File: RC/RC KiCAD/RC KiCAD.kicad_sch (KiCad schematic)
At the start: 10 parts, among them J1 USB_C_Receptacle_PowerOnly_6P, U1 MCP73871, U2 CR2013-MI2120

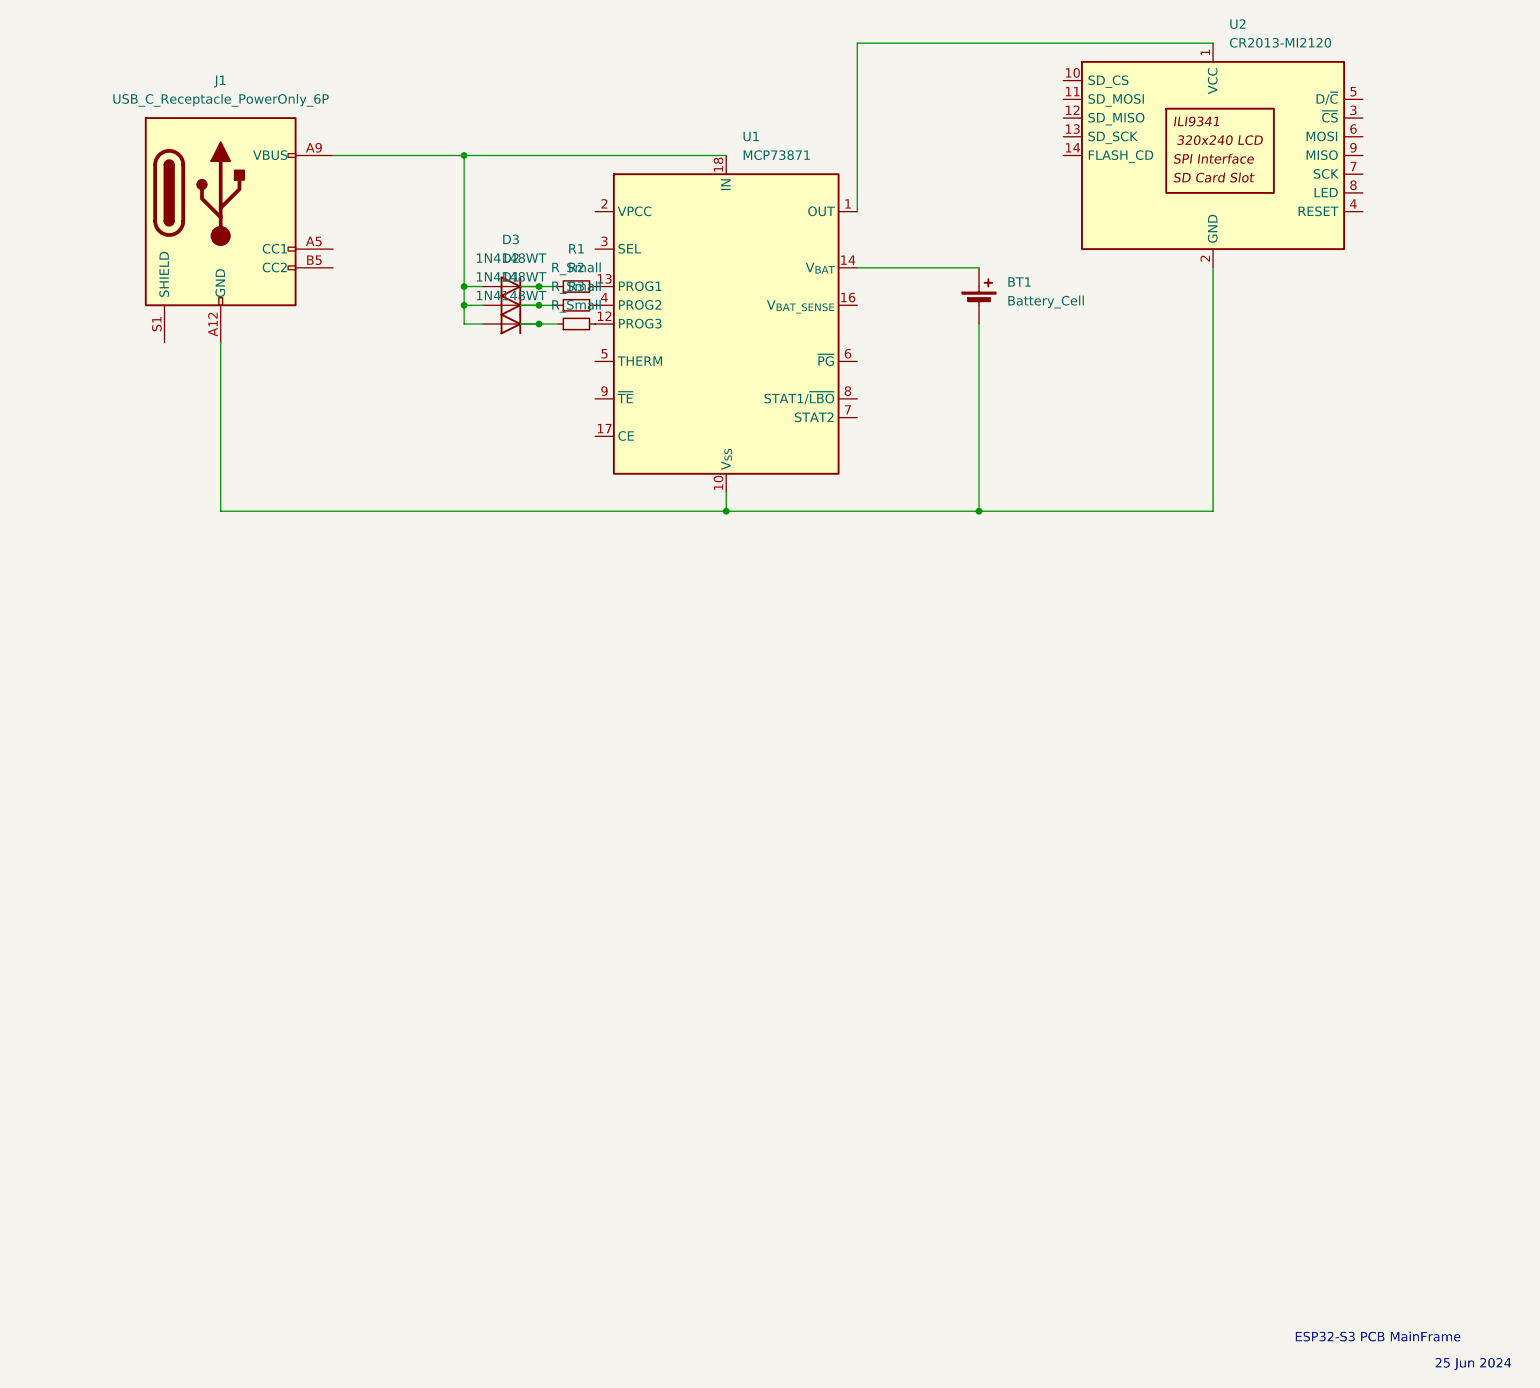
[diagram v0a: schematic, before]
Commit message: BMS FULL CAO
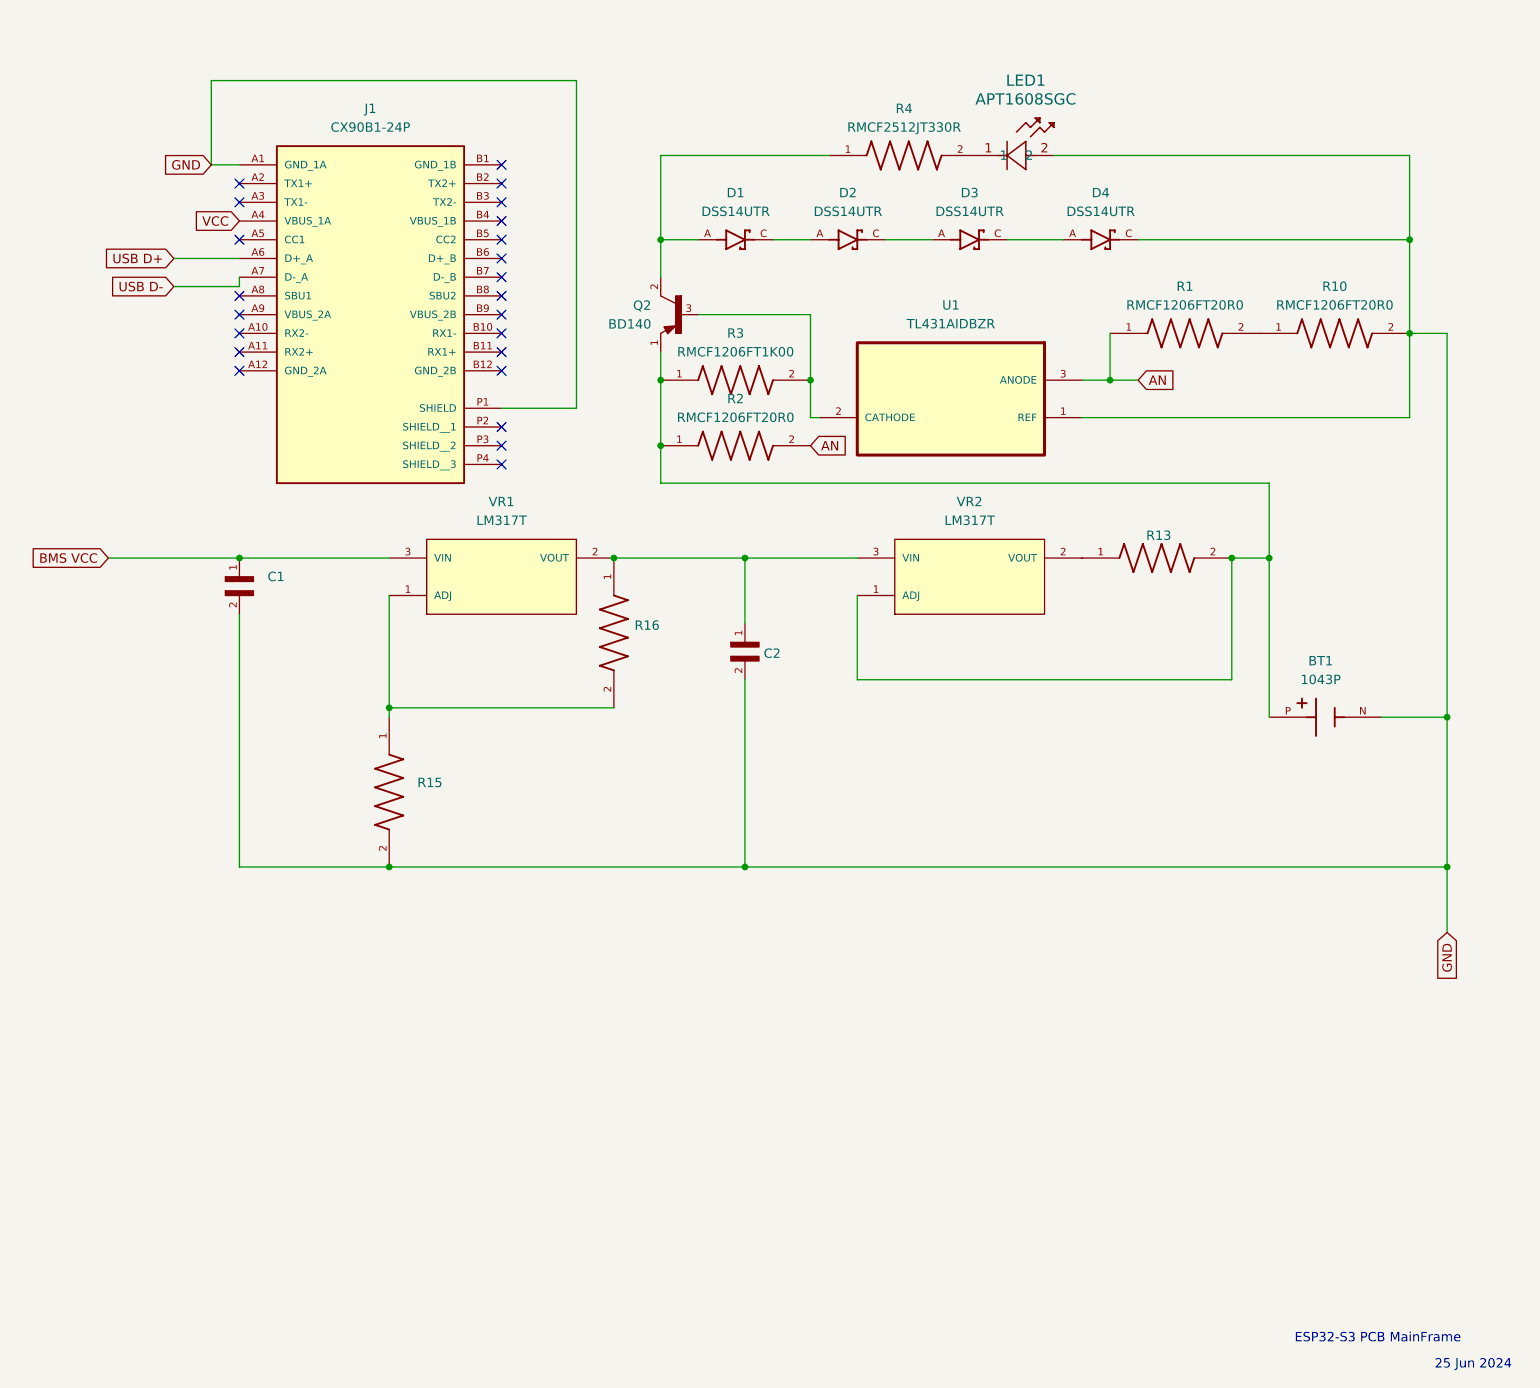
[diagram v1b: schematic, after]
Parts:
- removed BT1: Battery_Cell, Battery:BatteryHolder_MPD_BH-18650-PC2, symbol Device:Battery_Cell
- removed D1, D2, D3: 1N4148WT, Diode_SMD:D_SOD-523, symbol Diode:1N4148WT
- removed J1: USB_C_Receptacle_PowerOnly_6P, symbol Connector:USB_C_Receptacle_PowerOnly_6P
- removed R1, R2, R3: R_Small, Resistor_SMD:R_0201_0603Metric, symbol Device:R_Small
- removed U1: MCP73871, Package_DFN_QFN:QFN-20-1EP_4x4mm_P0.5mm_EP2.5x2.5mm, symbol Battery_Management:MCP73871
- removed U2: CR2013-MI2120, Display:CR2013-MI2120, symbol Driver_Display:CR2013-MI2120
- added BT1: 1043P, 1043P:BAT_1043P, symbol 1043P:1043P
- added C1, C2: JMK325ABJ107MM-P, JMK325ABJ107MM-P:CAPC3225X280N, symbol JMK325ABJ107MM-P:JMK325ABJ107MM-P
- added D1, D2, D3, D4: DSS14UTR, DSS14UTR:SODFL3618X110N, symbol DSS14UTR:DSS14UTR
- added J1: CX90B1-24P, CX90B1-24P:HRS_CX90B1-24P, symbol CX90B1-24P:CX90B1-24P
- added LED1: APT1608SGC, LED_APT1608SGC_KNB, symbol APT1608SGC:APT1608SGC
- added Q2: BD140, BD140:TO229P760X270X1364-3, symbol BD140:BD140
- added R1, R10, R2: RMCF1206FT20R0, RMCF1206FT20R0:RESC3216X70N, symbol RMCF1206FT20R0:RMCF1206FT20R0
- added R13: CRM2512-FX-2R00ELF, CRM2512_FX_2R00ELF:RESC6331X80N, symbol CRM2512-FX-2R00ELF:CRM2512-FX-2R00ELF
- added R15: RMCF2512JT3K30, RMCF2512JT3K30:RESC6332X70N, symbol RMCF2512JT3K30:RMCF2512JT3K30
- added R16: CRCW12101K40FKEA, CRCW12101K40FKEA:RESC3225X60N, symbol CRCW12101K40FKEA:CRCW12101K40FKEA
- added R3: RMCF1206FT1K00, RMCF1206FT1K00:RESC3216X70N, symbol RMCF1206FT1K00:RMCF1206FT1K00
- added R4: RMCF2512JT330R, RMCF2512JT330R:RESC6332X70N, symbol RMCF2512JT330R:RMCF2512JT330R
- added U1: TL431AIDBZR, TL431AIDBZR:SOT95P237X112-3N, symbol TL431AIDBZR:TL431AIDBZR
- added VR1, VR2: LM317T, LM317T:TO254P1054X470X1955-3, symbol LM317T:LM317T
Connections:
- new net: C2.1, R16.1, VR1.2 (VOUT), VR2.3 (VIN)
- new net: R15.1, R16.2, VR1.1 (ADJ)
- new net: D1.A, Q2.2, R4.1
- new net: LED1.1, R4.2
- new net: D2.C, D3.A
- new net: D3.C, D4.A
- new net: BT1.P, Q2.1, R13.2, R2.1, R3.1, VR2.1 (ADJ)
- new net: R13.1, VR2.2 (VOUT)
- new net: R1.2, R10.1
- new net: Q2.3, R3.2, U1.2 (CATHODE)
- new net: D1.C, D2.A
- new net AN: R1.1, R2.2, U1.3 (ANODE)
- new net BMS VCC: C1.1, VR1.3 (VIN)
- new net GND: BT1.N, C1.2, C2.2, D4.C, J1.A1 (GND_1A), J1.P1 (SHIELD), LED1.2, R10.2, R15.2, U1.1 (REF)
- new net USB D+: J1.A6 (D+_A)
- new net USB D-: J1.A7 (D-_A)
- new net VCC: J1.A4 (VBUS_1A)
- no-connect marks 0 -> 23
